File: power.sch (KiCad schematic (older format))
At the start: 25 parts, among them U201 LM1117-3.3, U202 LM1117-3.3, U203 LM1117-5.0, U204 STMPS2151

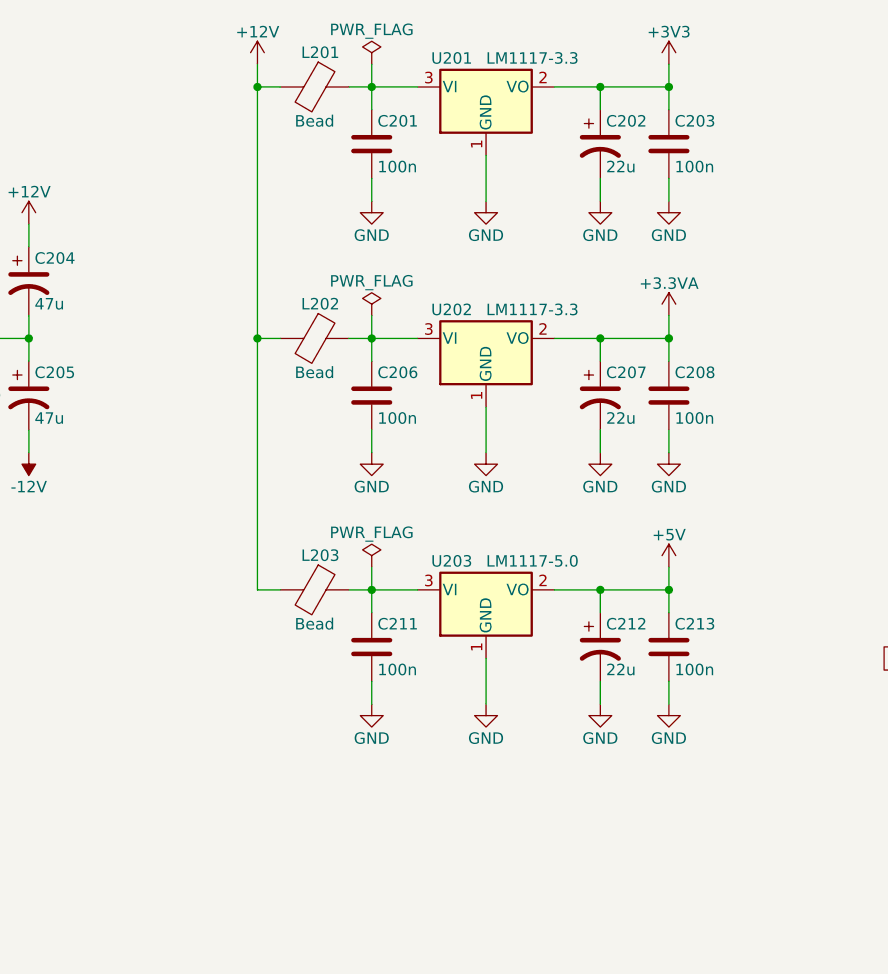
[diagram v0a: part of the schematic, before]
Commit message: work in progress
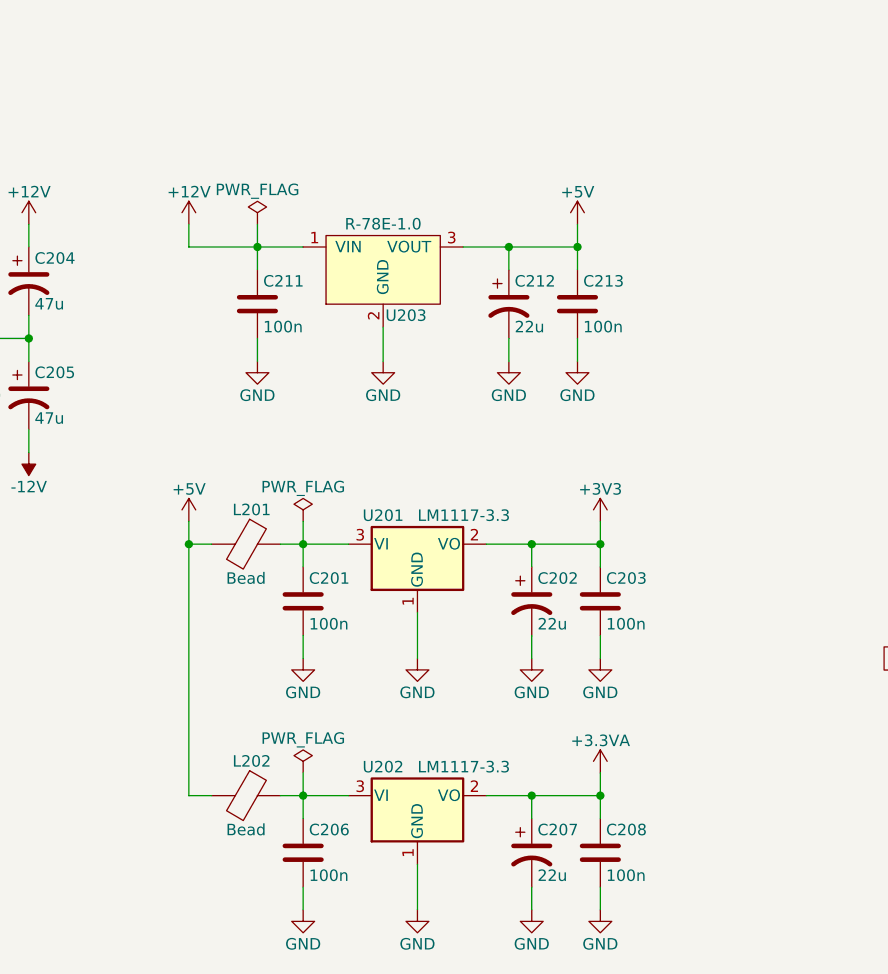
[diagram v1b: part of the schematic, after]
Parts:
- removed L203: Bead, Resistors_SMD:R_0603_HandSoldering, symbol Ferrite_Bead
- removed U203: LM1117-5.0, TO_SOT_Packages_SMD:SOT-223-3Lead_TabPin2, symbol LM1117-5.0
- added U203: R-78E-1.0, w_power:R-78E-1.0, symbol R-78E-1.0
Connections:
- net +12V: now also C211.1, U203.1 (VIN); no longer L201.2, L202.2
- net +5V: now also L201.2, L202.2, U203.3 (VOUT)
- net GND: now also U203.2 (GND)
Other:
- moved on the sheet: C201, C202, C203, C206, C207, C208, C211, C212, C213, L201, L202, U201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

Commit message: work in progress
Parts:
- C201, C203, C206, C208, C209, C211, C213: footprint Capacitors_SMD:C_0603_HandSoldering -> w_capacitor:C_0603
- L201, L202, R201, R203: footprint Resistors_SMD:R_0603_HandSoldering -> w_resistor:R_0603
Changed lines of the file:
@@
 F 0 "L201" V 4600 3725 50  0000 C CNN
 F 1 "Bead" V 4900 3700 50  0000 C CNN
-F 2 "Resistors_SMD:R_0603_HandSoldering" V 4680 3700 50  0001 C CNN
+F 2 "w_resistor:R_0603" V 4680 3700 50  0001 C CNN
 F 3 "http://datasheet.octopart.com/MI0603K300R-10-Steward-datasheet-14357321.pdf" H 4750 3700 50  0001 C CNN
 F 4 "Laird" H 4750 3700 60  0001 C CNN "MFN"
@@
 F 0 "C203" H 6325 4050 50  0000 L CNN
 F 1 "100n" H 6325 3850 50  0000 L CNN
-F 2 "Capacitors_SMD:C_0603_HandSoldering" H 6338 3800 50  0001 C CNN
+F 2 "w_capacitor:C_0603" H 6338 3800 50  0001 C CNN
 F 3 "http://datasheet.octopart.com/GRM188R71E104JA01J-Murata-datasheet-66077098.pdf" H 6300 3950 50  0001 C CNN
 F 4 "Murata" H 6325 4150 50  0001 C CNN "MFN"
@@
 F 0 "C208" H 6325 5150 50  0000 L CNN
 F 1 "100n" H 6325 4950 50  0000 L CNN
-F 2 "Capacitors_SMD:C_0603_HandSoldering" H 6338 4900 50  0001 C CNN
+F 2 "w_capacitor:C_0603" H 6338 4900 50  0001 C CNN
 F 3 "http://datasheet.octopart.com/GRM188R71E104JA01J-Murata-datasheet-66077098.pdf" H 6300 5050 50  0001 C CNN
 F 4 "Murata" H 6325 5250 50  0001 C CNN "MFN"
@@
 F 0 "C213" H 6225 2750 50  0000 L CNN
 F 1 "100n" H 6225 2550 50  0000 L CNN
-F 2 "Capacitors_SMD:C_0603_HandSoldering" H 6238 2500 50  0001 C CNN
+F 2 "w_capacitor:C_0603" H 6238 2500 50  0001 C CNN
 F 3 "http://datasheet.octopart.com/GRM188R71E104JA01J-Murata-datasheet-66077098.pdf" H 6200 2650 50  0001 C CNN
 F 4 "Murata" H 6225 2850 50  0001 C CNN "MFN"
@@
 F 0 "R201" V 7980 2550 50  0000 C CNN
 F 1 "1k" V 7900 2550 50  0000 C CNN
-F 2 "Resistors_SMD:R_0603_HandSoldering" V 7830 2550 50  0001 C CNN
+F 2 "w_resistor:R_0603" V 7830 2550 50  0001 C CNN
 F 3 "http://datasheet.octopart.com/ERJ-3EKF1001V-Panasonic-datasheet-82288794.pdf" H 7900 2550 50  0001 C CNN
 F 4 "Panasonic" H 7980 2650 50  0001 C CNN "MFN"
@@
 F 0 "C209" H 8225 3150 50  0000 L CNN
 F 1 "100n" H 8225 2950 50  0000 L CNN
-F 2 "Capacitors_SMD:C_0603_HandSoldering" H 8238 2900 50  0001 C CNN
+F 2 "w_capacitor:C_0603" H 8238 2900 50  0001 C CNN
 F 3 "http://datasheet.octopart.com/GRM188R71E104JA01J-Murata-datasheet-66077098.pdf" H 8200 3050 50  0001 C CNN
 F 4 "Murata" H 8225 3250 50  0001 C CNN "MFN"
@@
 F 0 "R203" V 8280 4450 50  0000 C CNN
 F 1 "10k" V 8200 4450 50  0000 C CNN
-F 2 "Resistors_SMD:R_0603_HandSoldering" V 8130 4450 50  0001 C CNN
+F 2 "w_resistor:R_0603" V 8130 4450 50  0001 C CNN
 F 3 "http://datasheet.octopart.com/ERJ-3EKF1002V-Panasonic-datasheet-13266541.pdf" H 8200 4450 50  0001 C CNN
 F 4 "Panasonic" H 8280 4550 50  0001 C CNN "MFN"
@@
 F 0 "L202" V 4600 4825 50  0000 C CNN
 F 1 "Bead" V 4900 4800 50  0000 C CNN
-F 2 "Resistors_SMD:R_0603_HandSoldering" V 4680 4800 50  0001 C CNN
+F 2 "w_resistor:R_0603" V 4680 4800 50  0001 C CNN
 F 3 "http://datasheet.octopart.com/MI0603K300R-10-Steward-datasheet-14357321.pdf" H 4750 4800 50  0001 C CNN
 F 4 "Laird" H 4750 4800 60  0001 C CNN "MFN"
@@
 F 0 "C201" H 5025 4050 50  0000 L CNN
 F 1 "100n" H 5025 3850 50  0000 L CNN
-F 2 "Capacitors_SMD:C_0603_HandSoldering" H 5038 3800 50  0001 C CNN
+F 2 "w_capacitor:C_0603" H 5038 3800 50  0001 C CNN
 F 3 "http://datasheet.octopart.com/GRM188R71E104JA01J-Murata-datasheet-66077098.pdf" H 5000 3950 50  0001 C CNN
 F 4 "Murata" H 5000 3950 60  0001 C CNN "MFN"
@@
 F 0 "C206" H 5025 5150 50  0000 L CNN
 F 1 "100n" H 5025 4950 50  0000 L CNN
-F 2 "Capacitors_SMD:C_0603_HandSoldering" H 5038 4900 50  0001 C CNN
+F 2 "w_capacitor:C_0603" H 5038 4900 50  0001 C CNN
 F 3 "http://datasheet.octopart.com/GRM188R71E104JA01J-Murata-datasheet-66077098.pdf" H 5000 5050 50  0001 C CNN
 F 4 "Murata" H 5000 5050 60  0001 C CNN "MFN"
@@
 F 0 "C211" H 4825 2750 50  0000 L CNN
 F 1 "100n" H 4825 2550 50  0000 L CNN
-F 2 "Capacitors_SMD:C_0603_HandSoldering" H 4838 2500 50  0001 C CNN
+F 2 "w_capacitor:C_0603" H 4838 2500 50  0001 C CNN
 F 3 "http://datasheet.octopart.com/GRM188R71E104JA01J-Murata-datasheet-66077098.pdf" H 4800 2650 50  0001 C CNN
 F 4 "Murata" H 4800 2650 60  0001 C CNN "MFN"

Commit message: cleanup
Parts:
- D201, D204: footprint Diodes_SMD:D_SOD-123 -> w_diode:D_SOD-123
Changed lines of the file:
@@
 F 0 "D201" H 1650 2700 50  0000 C CNN
 F 1 "1N5819HW" H 1650 2500 50  0000 C CNN
-F 2 "Diodes_SMD:D_SOD-123" H 1650 2600 50  0001 C CNN
+F 2 "w_diode:D_SOD-123" H 1650 2600 50  0001 C CNN
 F 3 "http://datasheet.octopart.com/1N5819HW-7-F-Diodes-Inc.-datasheet-34441420.pdf" H 1650 2600 50  0001 C CNN
 F 4 "Diodes Inc." H 1650 2800 50  0001 C CNN "MFN"
@@
 F 0 "D204" H 1650 3100 50  0000 C CNN
 F 1 "1N5819HW" H 1650 2900 50  0000 C CNN
-F 2 "Diodes_SMD:D_SOD-123" H 1650 3000 50  0001 C CNN
+F 2 "w_diode:D_SOD-123" H 1650 3000 50  0001 C CNN
 F 3 "http://datasheet.octopart.com/1N5819HW-7-F-Diodes-Inc.-datasheet-34441420.pdf" H 1650 3000 50  0001 C CNN
 F 4 "Diodes Inc." H 1650 3200 50  0001 C CNN "MFN"
